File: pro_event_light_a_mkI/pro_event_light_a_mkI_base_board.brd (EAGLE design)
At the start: 39.6 x 59.4 mm, 67 parts, among them K1 62201021121, P1-1:C10 10uF, P1-1:C2 220pF, P1-1:C3 45uF, P1-1:C4 4.7uF, P1-1:C6 4.7uF, P1-1:C7 4.7uF, P1-1:D1 MBR0540T1, P1-1:D3 1N4148WS, P1-1:L1 1uH, P1-1:R11 10K, P1-1:R12 17K5, P1-1:R13 27K, P1-1:U$4 LT1936, P2-1:DZ1 MBR0540T1, P2-1:L2 68uH, P2-1:PMIC1 ILD4001, P2-1:U1 PMXB56EN, SW1 ALPS_EC11D

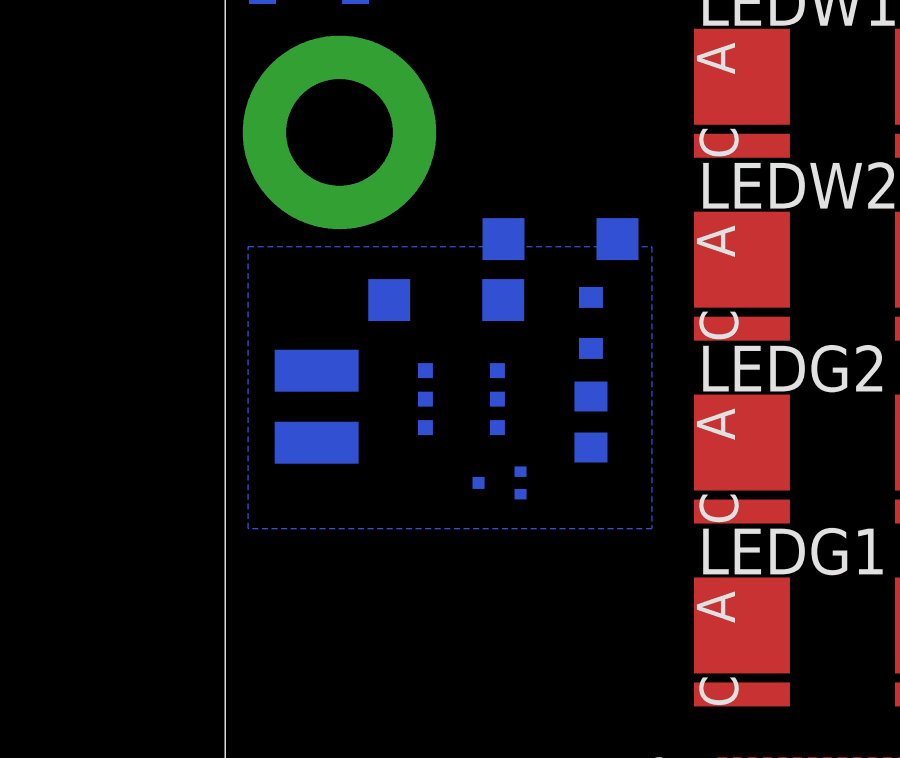
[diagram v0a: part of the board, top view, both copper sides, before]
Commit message: first layout of 4001
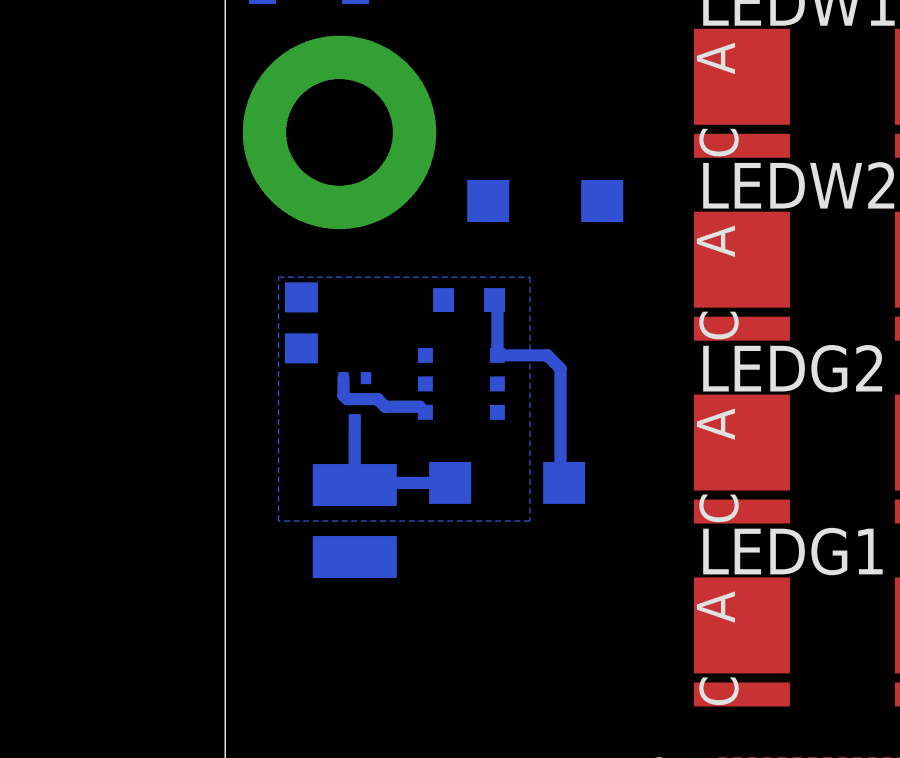
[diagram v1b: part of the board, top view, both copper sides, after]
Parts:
- moved P2-1:R14 10.2 mm to (2.54, 28.7)
- moved P2-1:DZ1 6.43 mm to (9.40, 23.4)
- moved P2-1:U1 5.58 mm to (4.32, 26.2), turned to 0 degrees
- moved P2-1:C8/1 4.13 mm to (8.13, 29.5), turned to 180 degrees
- moved P2-1:L2 4.02 mm to (4.32, 22.1)
- moved D2 1.37 mm to (10.7, 32.8)
- moved P2-1:PMIC1 0.51 mm to (7.87, 26.7)
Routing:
- net SUPPLY_24V: track 0.00 -> 8.01 mm
- net P2-1:N$29: track 0.00 -> 5.37 mm
- net P2-1:N$2: track 0.00 -> 3.54 mm
